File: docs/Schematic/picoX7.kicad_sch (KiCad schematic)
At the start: 34 parts, among them J1 MIDI in, J2 Debug, J3 Stereo line out, J4 Debug, SW1 RST, U1 MCU arm Cortex-M0x2, U2 I2S DAC, U3 H11L1, U4 74HCT164, U6 D1X8K-14BL, U7 D1X8K-14BL, U8 74HCT164

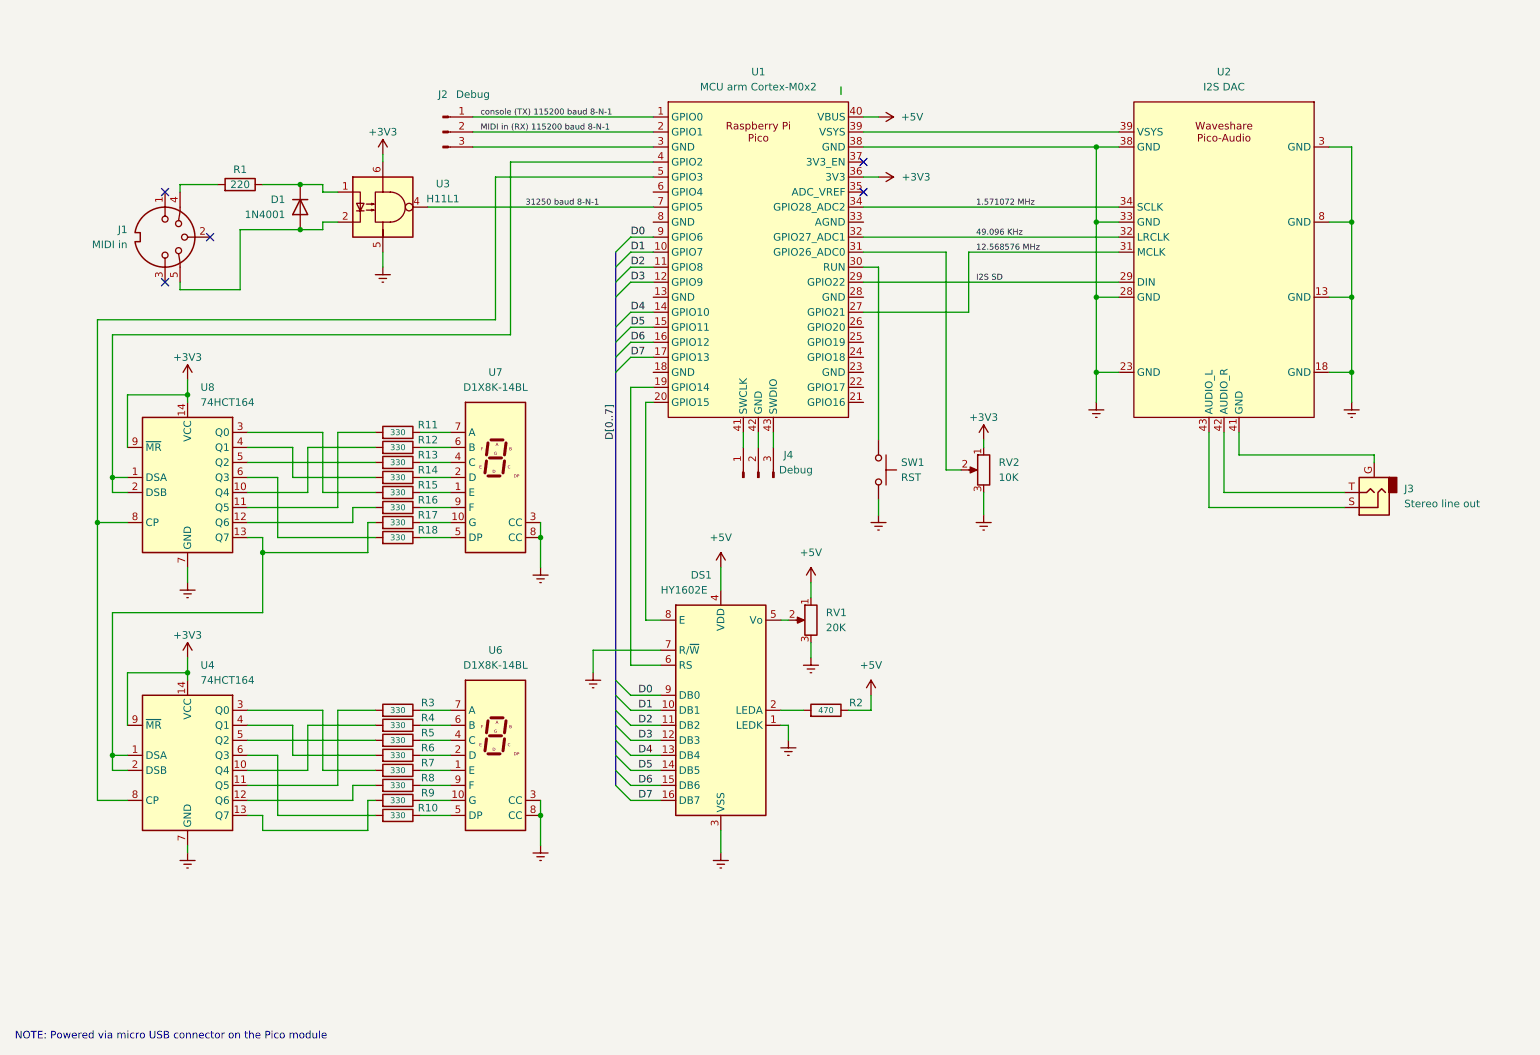
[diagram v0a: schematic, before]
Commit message: Updated schematic
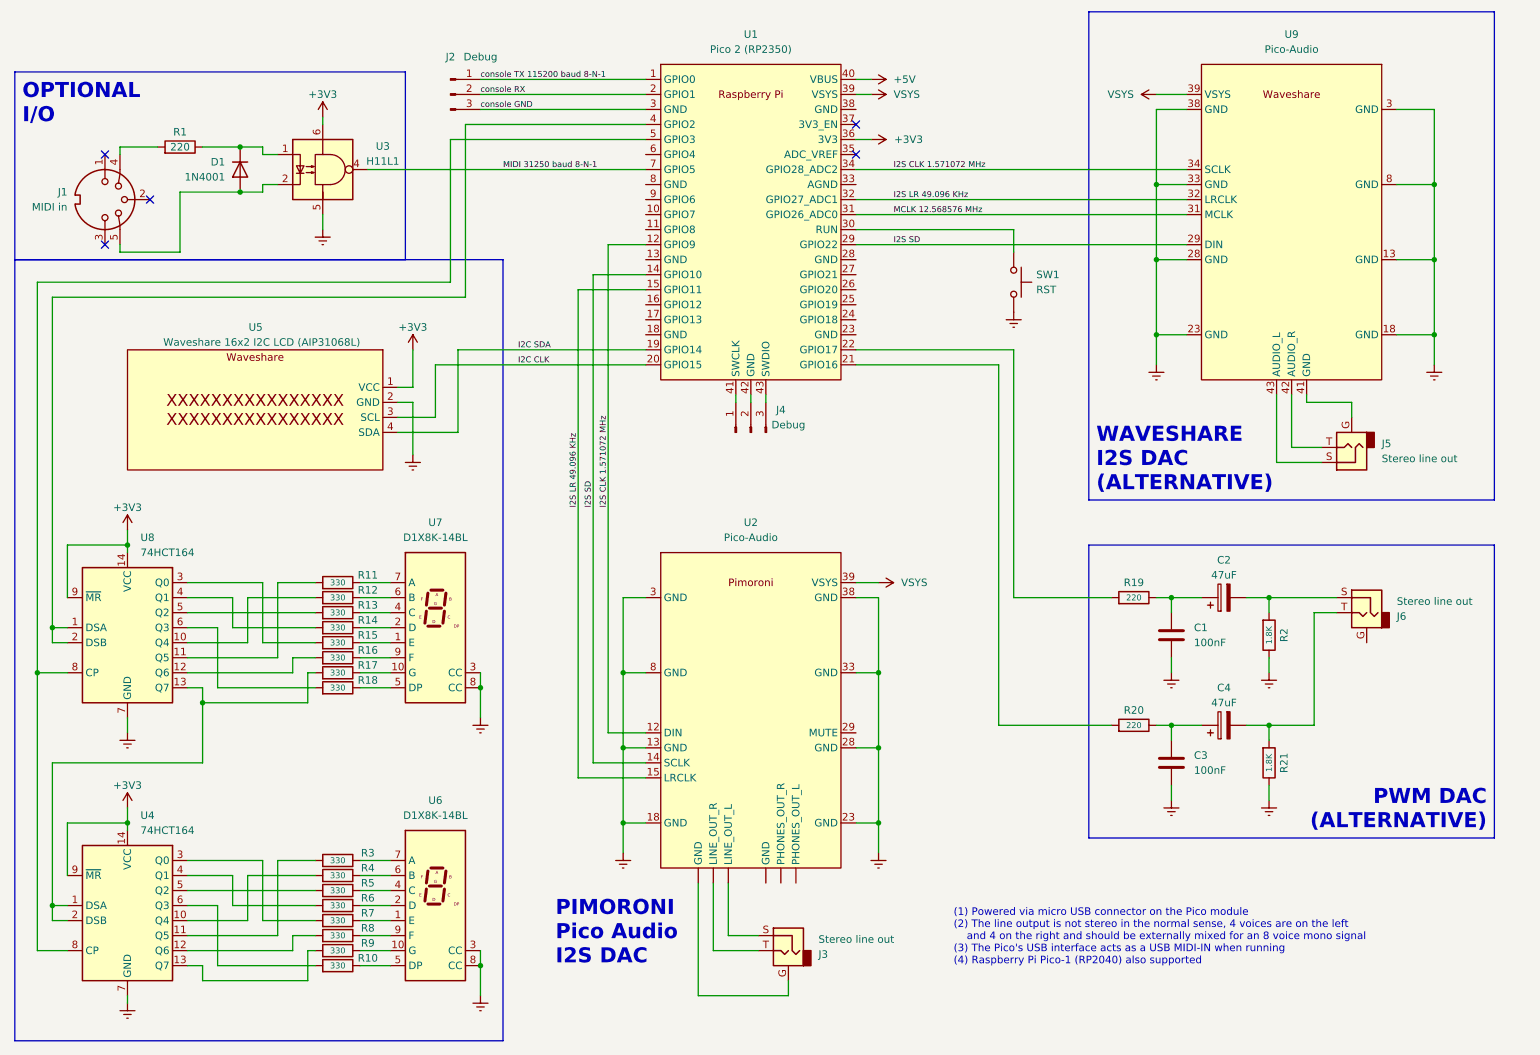
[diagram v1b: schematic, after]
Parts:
- removed DS1: HY1602E, Display:HY1602E, symbol Display_Character:HY1602E
- removed RV1: 20K, symbol Device:R_Potentiometer
- removed RV2: 10K, symbol Device:R_Potentiometer
- removed U1: MCU arm Cortex-M0x2, Package_DIP:DIP-40_W25.4mm_Socket_LongPads, symbol MCU_RaspberryPi_and_Boards:Pico
- removed U2: I2S DAC, Package_DIP:DIP-40_W25.4mm_Socket_LongPads, symbol MCU_RaspberryPi_and_Boards:Waveshare Pico-Audio
- added C1, C3: 100nF, symbol Device:C
- added C2, C4: 47uF, symbol Device:C_Polarized
- added J5, J6: Stereo line out, Connector_Audio:Jack_3.5mm_CUI_SJ1-3523N_Horizontal, symbol Connector_Audio:AudioJack2_Ground
- added R19, R20: 220, Resistor_THT:R_Axial_DIN0204_L3.6mm_D1.6mm_P5.08mm_Horizontal, symbol Device:R
- added R21: 1.8K, Resistor_THT:R_Axial_DIN0204_L3.6mm_D1.6mm_P5.08mm_Horizontal, symbol Device:R
- added U1: Pico 2 (RP2350), RPi_Pico:RPi_Pico_SMD_TH, symbol MCU_RaspberryPi_and_Boards:Pico 2
- added U2: Pico-Audio, RPi_Pico:RPi_Pico_SMD_TH, symbol MCU_RaspberryPi_and_Boards:Pimoroni Pico-Audio
- added U5: Waveshare 16x2 I2C LCD (AIP31068L), RPi_Pico:RPi_Pico_SMD_TH, symbol MCU_RaspberryPi_and_Boards:Waveshare 16x2 I2C LCD
- added U9: Pico-Audio, RPi_Pico:RPi_Pico_SMD_TH, symbol MCU_RaspberryPi_and_Boards:Waveshare Pico-Audio
- R2: value 470 -> 1.8K
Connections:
- net +3V3: now also U1.36 (3V3), U5.1 (VCC)
- net +5V: now also U1.39 (VSYS), U1.40 (VBUS), U2.39 (VSYS), U9.39 (VSYS); no longer R2.1
- net Earth: now also R2.1, C1.2, C3.2, R21.1, U2.13 (GND), U2.18 (GND), U2.23 (GND), U2.28 (GND), U2.3 (GND), U2.33 (GND), U2.38 (GND), U2.8 (GND), U5.2 (GND), U9.13 (GND), U9.18 (GND), U9.23 (GND), U9.28 (GND), U9.3 (GND), U9.33 (GND), U9.38 (GND), U9.8 (GND)
- net I2S SD: now also U1.14 (GPIO10), U1.29 (GPIO22), U2.14 (SCLK), U9.29 (DIN)
- net console GND: now reaches J2.3 (Pin_3)
- net console GND: now also U1.3 (GND)
- net at SW1.1: now also U1.30 (RUN)
- net at U8.1 (DSA), U8.2 (DSB): now also U1.4 (GPIO2)
- net at U4.8 (CP), U8.8 (CP): now also U1.5 (GPIO3)
- net at J3.G: now also U2. (PHONES_OUT_R)
- net at J3.S: now also U2. (PHONES_OUT_R)
- net at J3.T: now also U2. (PHONES_OUT_R)
- net at R2.2: now also C2.2, J6.S
- net at J4.1 (Pin_1): now also U1.41 (SWCLK)
- net at J4.2 (Pin_2): now also U1.42 (GND)
- net at J4.3 (Pin_3): now also U1.43 (SWDIO)
- net 31250 baud 8-N-1 renamed MIDI 31250 baud 8-N-1
- net MIDI 31250 baud 8-N-1: now also U1.7 (GPIO5)
- net MIDI in (RX) 115200 baud 8-N-1 renamed console RX
- net console RX: now also U1.2 (GPIO1)
- net console (TX) 115200 baud 8-N-1 renamed console TX 115200 baud 8-N-1 
- net console TX 115200 baud 8-N-1 : now also U1.1 (GPIO0)
- new net: R20.2, U1.21 (GPIO16)
- new net: R19.2, U1.22 (GPIO17)
- new net: C1.1, C2.1, R19.1
- new net: C3.1, C4.1, R20.1
- new net: C4.2, J6.T, R21.2
- new net: J5.G, U9.41 (GND)
- new net: J5.S, U9.43 (AUDIO_L)
- new net: J5.T, U9.42 (AUDIO_R)
- new net I2C CLK: U1.20 (GPIO15), U5.3 (SCL)
- new net I2C SDA: U1.19 (GPIO14), U5.4 (SDA)
- new net I2S CLK 1.571072 MHz: U1.12 (GPIO9), U1.34 (GPIO28_ADC2), U2.12 (DIN), U9.34 (SCLK)
- new net I2S LR 49.096 KHz: U1.15 (GPIO11), U1.32 (GPIO27_ADC1), U2.15 (LRCLK), U9.32 (LRCLK)
- new net MCLK 12.568576 MHz: U1.31 (GPIO26_ADC0), U9.31 (MCLK)
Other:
- note added: "(1) Powered via micro USB connector on the Pico module (2) The line output is not stereo in the normal sense, 4 voices are on the left and 4 on the right and should be externally mixed for an 8 voice mono signal (3) The Pico's USB interface acts as a USB MIDI-IN when running (4) Raspberry Pi Pico-1 (RP2040) also supported"
- note added: "OPTIONAL I/O"
- note added: "PIMORONI Pico Audio I2S DAC"
- note added: "PWM DAC (ALTERNATIVE)"
- note added: "WAVESHARE I2S DAC (ALTERNATIVE)"
- note removed: "NOTE: Powered via micro USB connector on the Pico module"
- moved on the sheet: D1, J1, J2, J3, J4, R1, R10, R11, R12, R13, R14, R15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
